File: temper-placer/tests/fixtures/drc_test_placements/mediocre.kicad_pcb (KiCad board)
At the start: 2 copper layers, 50 x 30 mm, 4 parts, among them U1 LM358

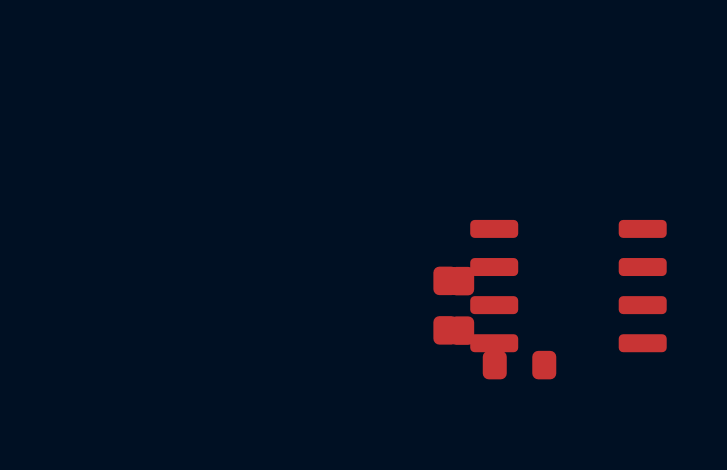
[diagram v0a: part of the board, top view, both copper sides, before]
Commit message: merge for sharing
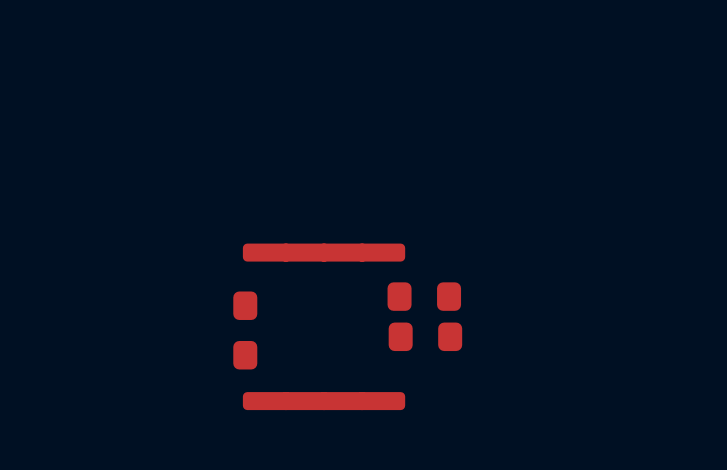
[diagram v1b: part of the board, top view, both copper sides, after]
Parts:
- moved U1 8.26 mm to (202.4, 153.4), turned to 90 degrees
- moved R1 6.72 mm to (199.7, 153.5)
- moved R2 3.28 mm to (205.8, 153.7)
- moved C1 1.30 mm to (205.7, 152.4), turned to 0 degrees
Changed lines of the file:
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@@
   (net 4 "SIG2")
   (footprint "Resistor_SMD:R_0603_1608Metric" (layer "F.Cu")
-    (at 206.41836324481005 152.68757851138673 90.0)
+    (at 199.748772873673 153.51630763178667 90.0)
     (property "Reference" "R1")
     (property "Value" "10k")
@@
   )
   (footprint "Resistor_SMD:R_0603_1608Metric" (layer "F.Cu")
-    (at 208.8896784186639 154.6703525716194 0.0)
+    (at 205.7534685396509 153.72662510139173 0.0)
     (property "Reference" "R2")
     (property "Value" "4.7k")
@@
   )
   (footprint "Capacitor_SMD:C_0603_1608Metric" (layer "F.Cu")
-    (at 206.978517025568 152.69584222732271 90.0)
+    (at 205.71572434426218 152.38670351602337 0.0)
     (property "Reference" "C1")
     (property "Value" "100nF")
@@
   )
   (footprint "Package_SO:SOIC-8_3.9x4.9mm_P1.27mm" (layer "F.Cu")
-    (at 210.52108022846065 152.03580369594079 0.0)
+    (at 202.37346147158888 153.3943308817871 90.0)
     (property "Reference" "U1")
     (property "Value" "LM358")
